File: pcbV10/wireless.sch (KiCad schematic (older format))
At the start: 7 parts, among them J14 LoRa Antenna, U16 MODULE_STEPDOWN, U17 RFM95W-868S2

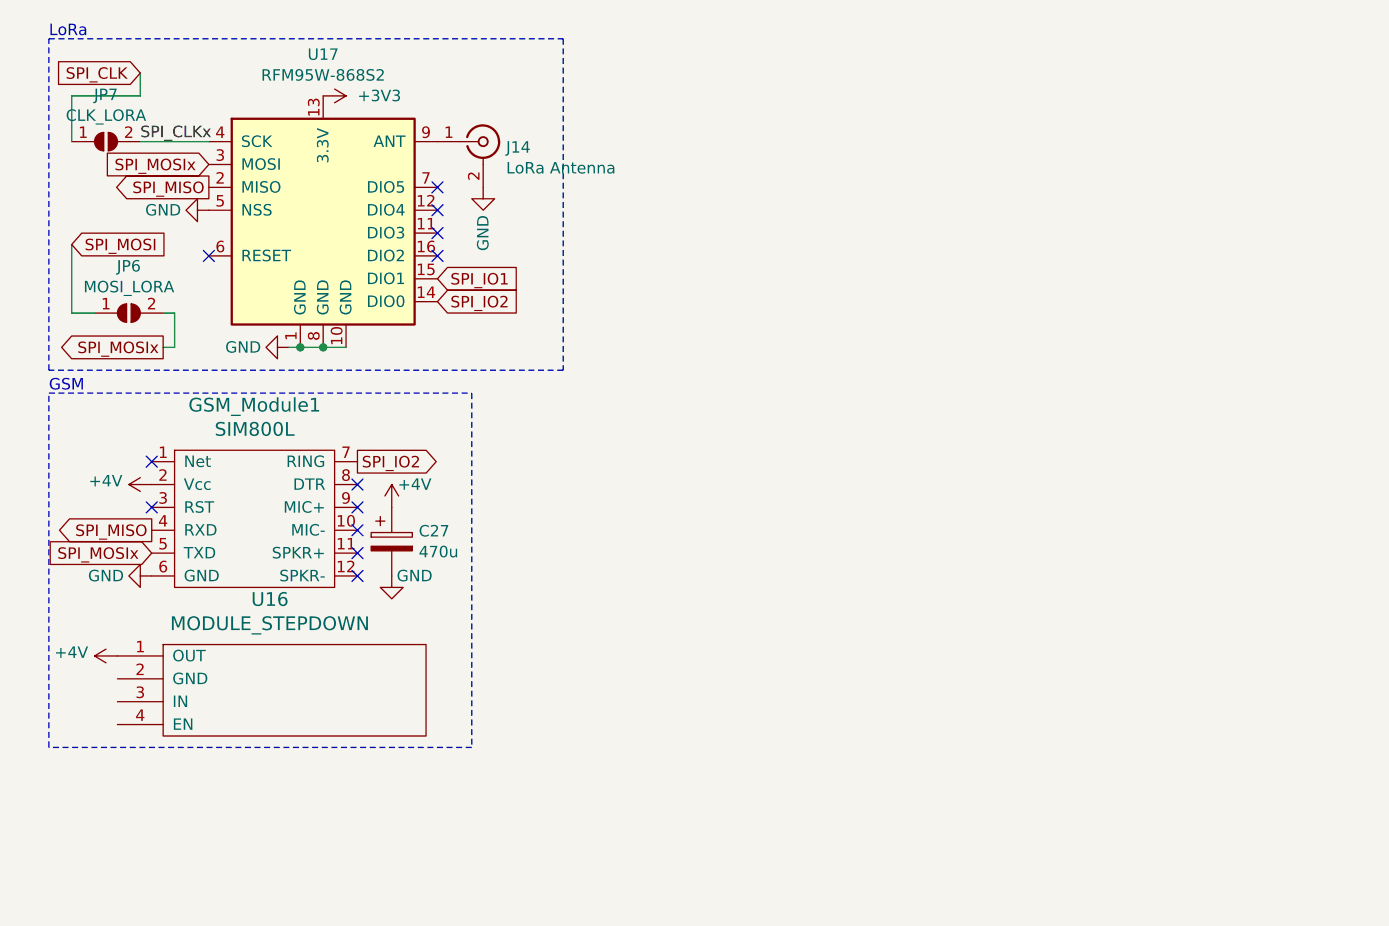
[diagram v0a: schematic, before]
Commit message: labathome v11 as ordered @ JLCPCB
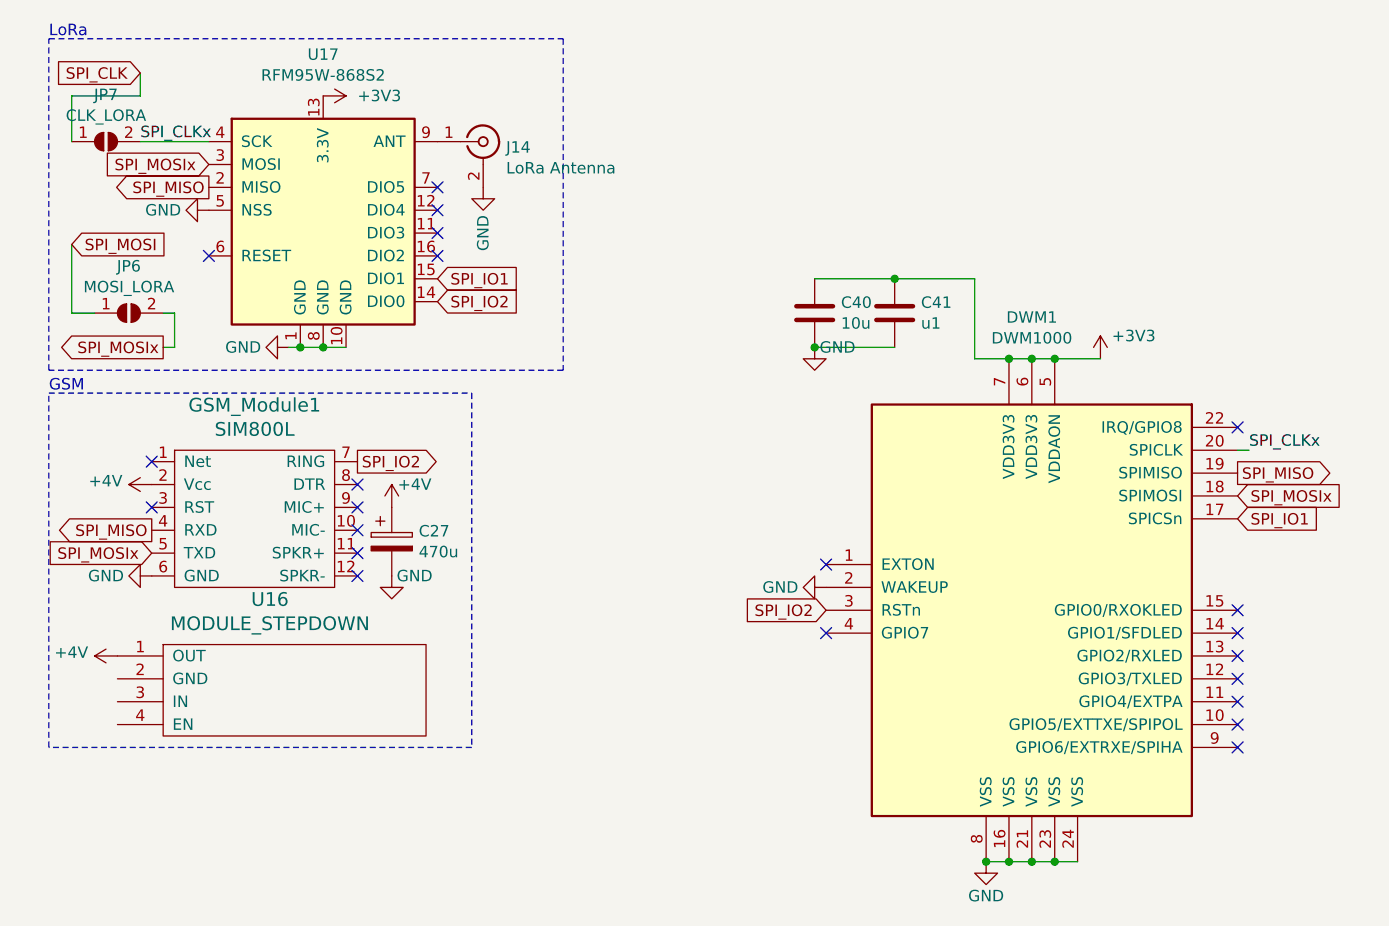
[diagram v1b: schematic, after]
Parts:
- added C40: 10u, Capacitor_SMD:C_0805_2012Metric_Pad1.18x1.45mm_HandSolder, symbol Device:C
- added C41: u1, Capacitor_SMD:C_0805_2012Metric_Pad1.18x1.45mm_HandSolder, symbol Device:C
- added DWM1: DWM1000, RF_Module:DWM1000, symbol RF_Module:DWM1000
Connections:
- net +3V3: now also C40.1, C41.1, DWM1.5 (VDDAON), DWM1.6 (VDD3V3), DWM1.7 (VDD3V3)
- net GND: now also C40.2, C41.2, DWM1.16 (VSS), DWM1.2 (WAKEUP), DWM1.21 (VSS), DWM1.23 (VSS), DWM1.24 (VSS), DWM1.8 (VSS)
- net SPI_CLKx: now also DWM1.20 (SPICLK)
- net SPI_IO1: now also DWM1.17 (SPICSn)
- net SPI_IO2: now also DWM1.3 (RSTn)
- net SPI_MISO: now also DWM1.19 (SPIMISO)
- net SPI_MOSIx: now also DWM1.18 (SPIMOSI)
- no-connect marks 12 -> 22
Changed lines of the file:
@@
 $Descr A4 11693 8268
 encoding utf-8
-Sheet 3 4
+Sheet 3 5
 Title ""
 Date ""
@@
 Text Label 1000 1050 0    50   ~ 0
 SPI_CLKx
+$Comp
+L RF_Module:DWM1000 DWM?
+U 1 1 61C6ED51
+P 4900 3100
+AR Path="/61D72F6F/61C6ED51" Ref="DWM?"  Part="1"
+AR Path="/622D65C1/61C6ED51" Ref="DWM1"  Part="1"
+F 0 "DWM1" H 4900 4381 50  0000 C CNN
+F 1 "DWM1000" H 4900 4290 50  0000 C CNN
+F 2 "RF_Module:DWM1000" H 5600 2100 50  0001 C CNN
+F 3 "https://www.decawave.com/sites/default/files/resources/dwm1000-datasheet-v1.3.pdf" H 7300 2000 50  0001 C CNN
+	1    4900 3100
+	1    0    0    -1
+$EndComp
+$Comp
+L power:+3V3 #PWR?
+U 1 1 61C6ED57
+P 5200 2000
+AR Path="/61D72F6F/61C6ED57" Ref="#PWR?"  Part="1"
+AR Path="/622D65C1/61C6ED57" Ref="#PWR0136"  Part="1"
+F 0 "#PWR0136" H 5200 1850 50  0001 C CNN
+F 1 "+3V3" H 5250 2100 50  0000 L CNN
+F 2 "" H 5200 2000 50  0001 C CNN
+F 3 "" H 5200 2000 50  0001 C CNN
+	1    5200 2000
+	1    0    0    -1
+$EndComp
+Wire Wire Line
+	4800 2000 4900 2000
+Connection ~ 4900 2000
+Wire Wire Line
+	4900 2000 5000 2000
+Connection ~ 5000 2000
+Wire Wire Line
+	5000 2000 5200 2000
+Text GLabel 5800 2600 2    50   Input ~ 0
+SPI_MOSIx
+Text GLabel 5800 2500 2    50   Output ~ 0
+SPI_MISO
+Text Label 5850 2400 0    50   ~ 0
+SPI_CLKx
+Wire Wire Line
+	5800 2400 5850 2400
+Text GLabel 5800 2700 2    50   Input ~ 0
+SPI_IO1
+Text GLabel 4000 3100 0    50   Input ~ 0
+SPI_IO2
+NoConn ~ 4000 2900
+NoConn ~ 4000 3200
+NoConn ~ 5800 2300
+NoConn ~ 5800 3700
+NoConn ~ 5800 3600
+NoConn ~ 5800 3500
+NoConn ~ 5800 3400
+NoConn ~ 5800 3300
+NoConn ~ 5800 3200
+NoConn ~ 5800 3100
+$Comp
+L power:GND #PWR0137
+U 1 1 61C74709
+P 4700 4200
+F 0 "#PWR0137" H 4700 3950 50  0001 C CNN
+F 1 "GND" H 4700 4050 50  0000 C CNN
+F 2 "" H 4700 4200 50  0001 C CNN
+F 3 "" H 4700 4200 50  0001 C CNN
+	1    4700 4200
+	1    0    0    -1
+$EndComp
+Wire Wire Line
+	5100 4200 5000 4200
+Connection ~ 4700 4200
+Connection ~ 4800 4200
+Wire Wire Line
+	4800 4200 4700 4200
+Connection ~ 4900 4200
+Wire Wire Line
+	4900 4200 4800 4200
+Connection ~ 5000 4200
+Wire Wire Line
+	5000 4200 4900 4200
+$Comp
+L power:GND #PWR0139
+U 1 1 61C7544D
+P 4000 3000
+F 0 "#PWR0139" H 4000 2750 50  0001 C CNN
+F 1 "GND" V 4000 2800 50  0000 C CNN
+F 2 "" H 4000 3000 50  0001 C CNN
+F 3 "" H 4000 3000 50  0001 C CNN
+	1    4000 3000
+	0    1    1    0
+$EndComp
+$Comp
+L Device:C C41
+U 1 1 61C41063
+P 4300 1800
+F 0 "C41" H 4415 1846 50  0000 L CNN
+F 1 "u1" H 4415 1755 50  0000 L CNN
+F 2 "Capacitor_SMD:C_0805_2012Metric_Pad1.18x1.45mm_HandSolder" H 4338 1650 50  0001 C CNN
+F 3 "~" H 4300 1800 50  0001 C CNN
+	1    4300 1800
+	1    0    0    -1
+$EndComp
+$Comp
+L Device:C C40
+U 1 1 61C41A80
+P 3950 1800
+F 0 "C40" H 4065 1846 50  0000 L CNN
+F 1 "10u" H 4065 1755 50  0000 L CNN
+F 2 "Capacitor_SMD:C_0805_2012Metric_Pad1.18x1.45mm_HandSolder" H 3988 1650 50  0001 C CNN
+F 3 "~" H 3950 1800 50  0001 C CNN
+	1    3950 1800
+	1    0    0    -1
+$EndComp
+Wire Wire Line
+	4800 2000 4650 2000
+Wire Wire Line
+	4650 2000 4650 1650
+Wire Wire Line
+	4650 1650 4300 1650
+Connection ~ 4800 2000
+Wire Wire Line
+	3950 1650 4300 1650
+Connection ~ 4300 1650
+Wire Wire Line
+	3950 1950 4300 1950
+$Comp
+L power:GND #PWR055
+U 1 1 61C42E11
+P 3950 1950
+F 0 "#PWR055" H 3950 1700 50  0001 C CNN
+F 1 "GND" H 4050 1950 50  0000 C CNN
+F 2 "" H 3950 1950 50  0001 C CNN
+F 3 "" H 3950 1950 50  0001 C CNN
+	1    3950 1950
+	1    0    0    -1
+$EndComp
+Connection ~ 3950 1950
 $EndSCHEMATC
